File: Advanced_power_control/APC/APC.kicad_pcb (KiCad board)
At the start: 4 copper layers, 65 x 100 mm, 50 parts, among them J1 AVR-JTAG-10, J10 CMD_IN, J11 PWR_V_SEL, J12 12/24 V_IN, J13 220_OUT, J2 EM_STOP_INT, J3 STATUS_LED, J4 EM_STOP, J5 POWER_BUTTON, J6 POWER_LED, J7 220 IN, J8 CMD_OUT, J9 CMD_V_SEL, K1 G5LE-1, Q1 IRLML0030, Q2 IRLML0030, Q3 IRLML0030, U1 ATmega164PA-AU, U2 LTV-817, U3 LTV-817, U4 LTV-817

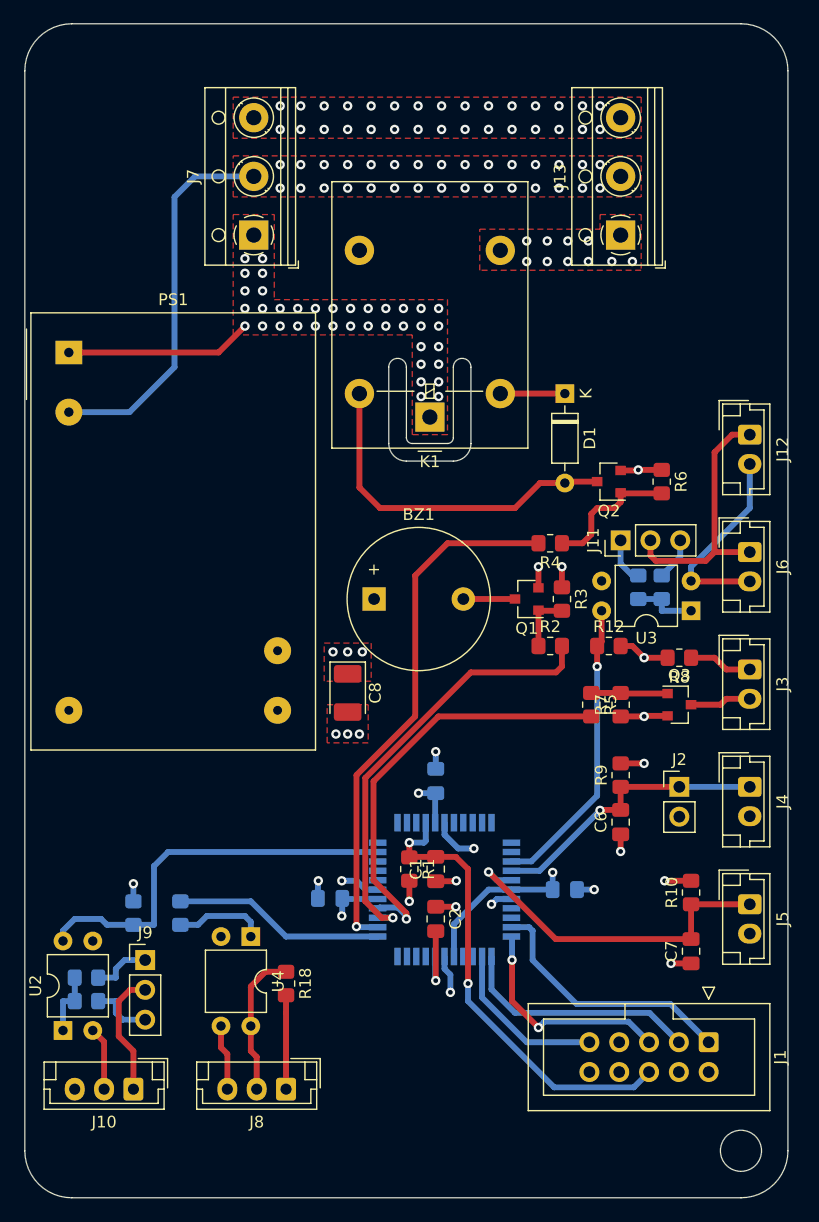
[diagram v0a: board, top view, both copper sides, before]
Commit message: update schematic and board
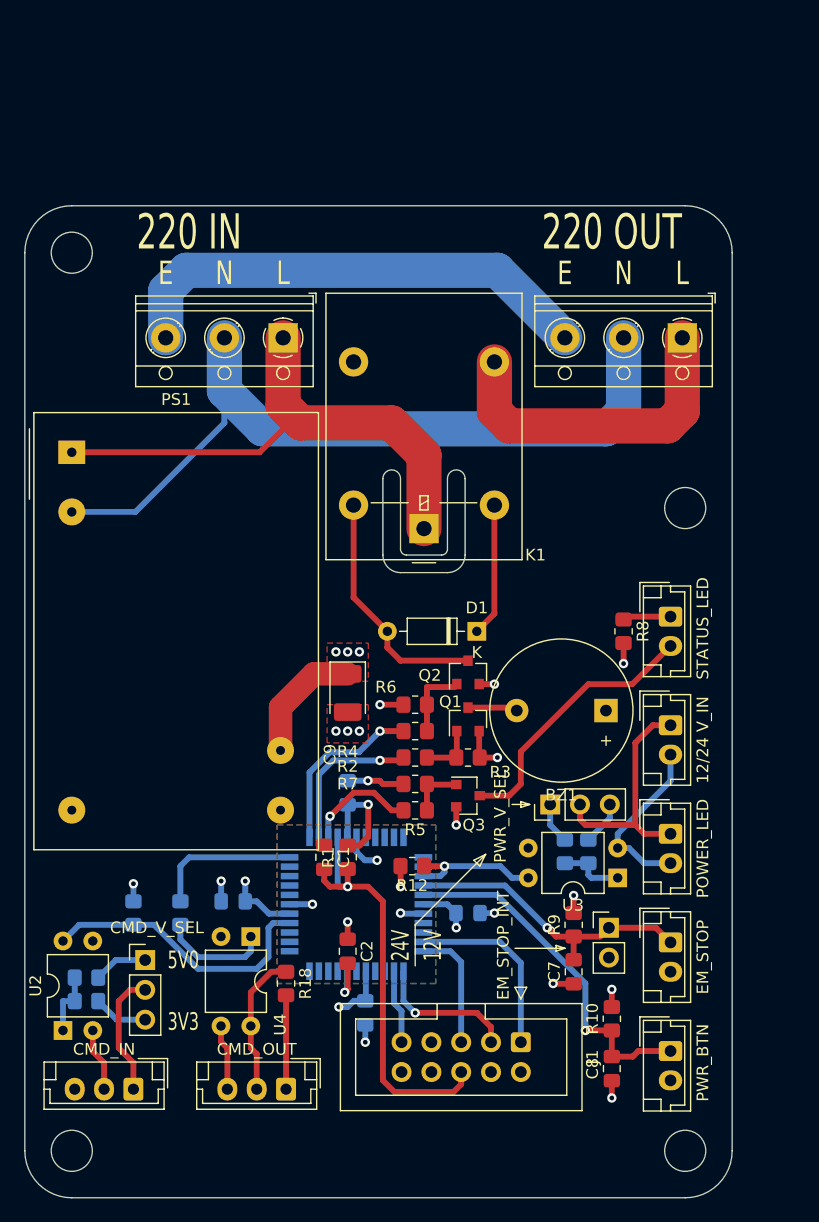
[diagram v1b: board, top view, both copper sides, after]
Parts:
- added C6: 0.1uF, Capacitor_SMD:C_0805_2012Metric_Pad1.15x1.40mm_HandSolder, B.Cu at (115.2, 91.2)
- C1, C2, C3, C4, C5: footprint Capacitor_SMD:C_0805_2012Metric_Pad1.18x1.45mm_HandSolder -> Capacitor_SMD:C_0805_2012Metric_Pad1.15x1.40mm_HandSolder
- C7: renamed from C6; footprint Capacitor_SMD:C_0805_2012Metric_Pad1.18x1.45mm_HandSolder -> Capacitor_SMD:C_0805_2012Metric_Pad1.15x1.40mm_HandSolder
- C8: renamed from C7; footprint Capacitor_SMD:C_0805_2012Metric_Pad1.18x1.45mm_HandSolder -> Capacitor_SMD:C_0805_2012Metric_Pad1.15x1.40mm_HandSolder
- J13: value 220_OUT -> 220 OUT
- J5: value POWER_BUTTON -> PWR_BTN
- moved R6 28.3 mm to (119.5, 65.0), turned to 0 degrees
- moved J12 25.7 mm to (141.2, 66.8)
- moved R12 25.1 mm to (119.2, 78.8), turned to 180 degrees
- moved J6 24.9 mm to (141.2, 76.0)
- moved U3 23.6 mm to (136.8, 79.8)
- moved R16 23.4 mm to (134.2, 77.5)
- moved R17 23.4 mm to (132.2, 77.5)
- moved J11 23.3 mm to (131.0, 73.5)
- moved BZ1 21.9 mm to (135.8, 65.5), turned to 180 degrees
- moved D1 21.6 mm to (124.8, 58.8), turned to 180 degrees
- moved Q2 20.2 mm to (124.0, 62.2), turned to 90 degrees
- moved R4 19.7 mm to (119.5, 67.2)
- moved Q3 19.6 mm to (124.0, 72.8)
- moved R7 18.8 mm to (119.5, 71.8), turned to 0 degrees
- moved R5 17.5 mm to (119.5, 74.0), turned to 180 degrees
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- renumbered C8 to C9
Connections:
- U1 pad 1: (no net) -> /PWR
- U1 pad 2: (no net) -> /S_STATE
- U1 pad 3: (no net) -> /STATE
- U1 pad 34: /CMD_OUT -> (no net)
- U1 pad 35: /PWR -> (no net)
- U1 pad 36: /S_STATE -> (no net)
- U1 pad 37: /STATE -> /CMD_IN
- U1 pad 43: /CMD_IN -> (no net)
- U1 pad 44: (no net) -> /CMD_OUT
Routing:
- net /E: track 0.00 -> 41.1 mm, vias 30 -> 0
- net +5V: track 236.3 -> 197.9 mm, vias 11 -> 12
- net /N: track 32.6 -> 70.1 mm, vias 30 -> 0
- net /L_I: track 15.9 -> 52.3 mm, vias 38 -> 0
- net /PWR: track 45.4 -> 15.0 mm
- net /L_O: track 0.00 -> 27.5 mm, vias 10 -> 0
- net /STATE: track 36.8 -> 9.56 mm
- net /S_STATE: track 37.2 -> 13.1 mm
- net Net-(J3-Pad2): track 5.21 -> 23.1 mm
- net /V_IN_DET: track 25.5 -> 11.7 mm
- net /CMD_IN: track 33.8 -> 24.5 mm
- net /P_ON: track 29.9 -> 20.7 mm
- net /TMS: track 19.1 -> 10.4 mm, vias 2 -> 0
- net /TDO: track 20.6 -> 12.2 mm, vias 0 -> 1
- net /TDI: track 14.2 -> 6.32 mm
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- added copper zone on B.Cu, net GND
- removed copper zone on F.Cu, net /E
- removed copper zone on F.Cu, net /L_I
- removed copper zone on F.Cu, net /L_O
- removed copper zone on F.Cu, net /N
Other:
- board size 65 x 100 mm -> 60.2 x 84.5 mm
- board text added: "12V"
- board text added: "24V"
- board text added: "3V3"
- board text added: "5V0"
- board text added: "E"
- board text added: "L"
- board text added: "N"
